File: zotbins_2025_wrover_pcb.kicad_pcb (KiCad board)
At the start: 2 copper layers, 107 x 98 mm, 26 parts

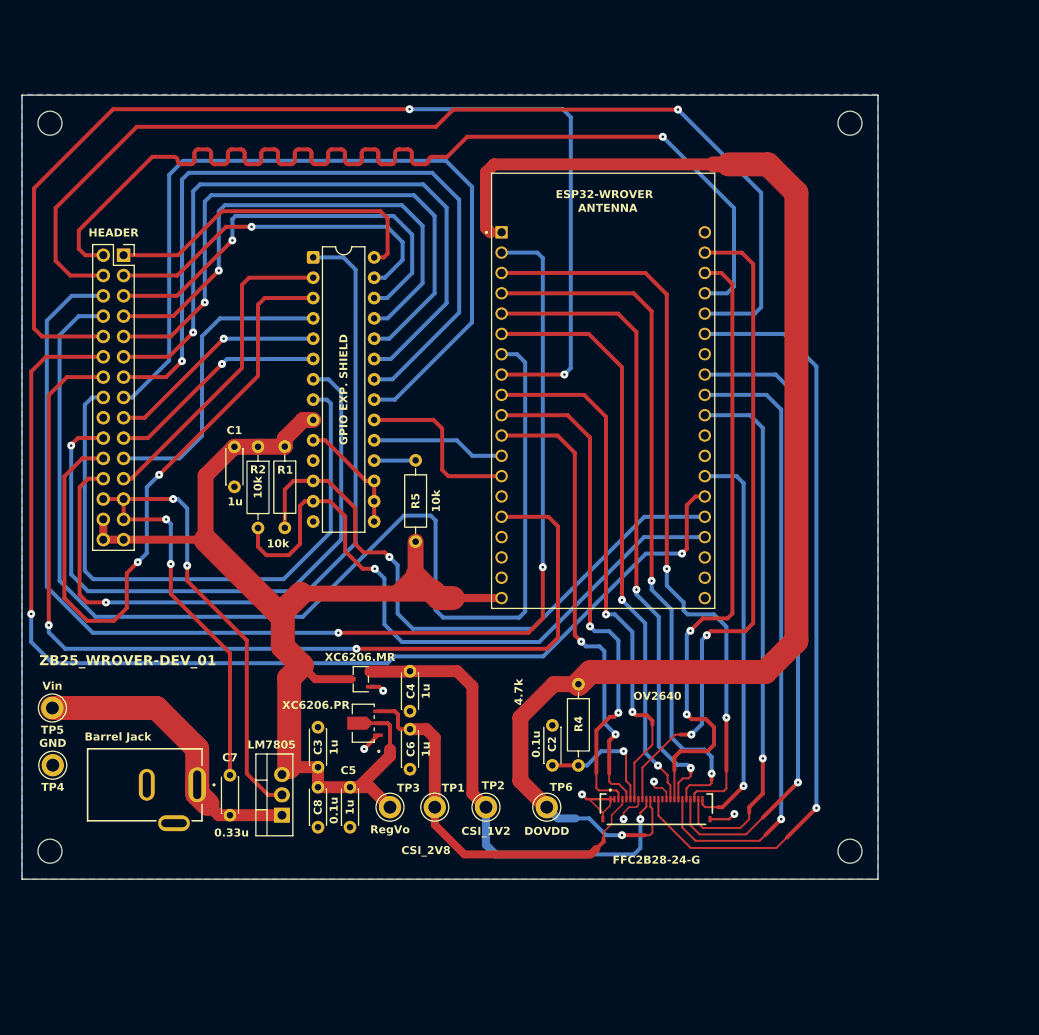
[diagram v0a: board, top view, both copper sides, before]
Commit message: basically the final version; just final adjustments with labeling and silkscreen needed. Traces, all components are all set.
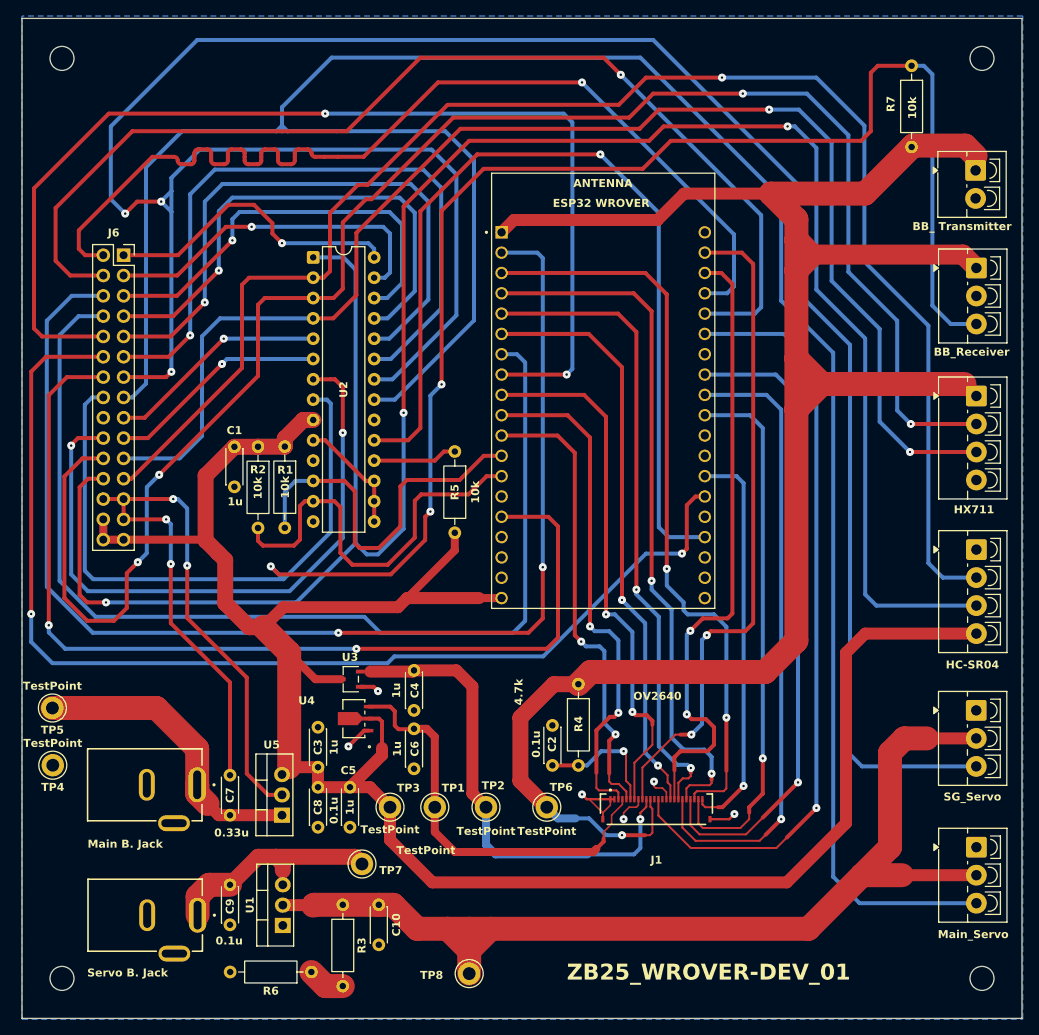
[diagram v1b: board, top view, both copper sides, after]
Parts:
- added BB_ Transmitter: BB_Transmitter_Screw_Terminal_01x02, TerminalBlock_4Ucon:TerminalBlock_4Ucon_1x02_P3.50mm_Vertical, F.Cu at (212.2, 56.4)
- added BB_Receiver: BB_Receiver_Screw_Terminal_01x03, TerminalBlock_4Ucon:TerminalBlock_4Ucon_1x03_P3.50mm_Vertical, F.Cu at (212.3, 68.6)
- added C10: 1u, Capacitor_THT:C_Disc_D4.3mm_W1.9mm_P5.00mm, F.Cu at (137.6, 148.2)
- added C9: 0.1u, Capacitor_THT:C_Disc_D4.3mm_W1.9mm_P5.00mm, F.Cu at (119.0, 145.7)
- added HC-SR04: HC-SR04_Screw_Terminal_01x04, TerminalBlock_4Ucon:TerminalBlock_4Ucon_1x04_P3.50mm_Vertical, F.Cu at (212.3, 103.8)
- added HX711: HX711_Screw_Terminal_01x04, TerminalBlock_4Ucon:TerminalBlock_4Ucon_1x04_P3.50mm_Vertical, F.Cu at (212.3, 84.6)
- added Main_Servo: Main_Servo_Screw_Terminal_01x03, TerminalBlock_4Ucon:TerminalBlock_4Ucon_1x03_P3.50mm_Vertical, F.Cu at (212.3, 141.0)
- added R3: 240, Resistor_THT:R_Axial_DIN0207_L6.3mm_D2.5mm_P10.16mm_Horizontal, F.Cu at (133.1, 148.2)
- added R6: 800, Resistor_THT:R_Axial_DIN0207_L6.3mm_D2.5mm_P10.16mm_Horizontal, F.Cu at (129.2, 156.6)
- added R7: 10k, Resistor_THT:R_Axial_DIN0207_L6.3mm_D2.5mm_P10.16mm_Horizontal, F.Cu at (204.2, 43.3)
- added SG_Servo: SG_Servo_Screw_Terminal_01x03, TerminalBlock_4Ucon:TerminalBlock_4Ucon_1x03_P3.50mm_Vertical, F.Cu at (212.3, 123.9)
- added Servo B. Jack: DCJ200-10-A-XX-K_REVA, Library:GCT_DCJ200-10-A-XX-K_REVA, F.Cu at (108.4, 149.5)
- added TP7: TestPoint, TestPoint:TestPoint_Keystone_5005-5009_Compact, F.Cu at (135.5, 143.1)
- added TP8: TestPoint, TestPoint:TestPoint_Keystone_5005-5009_Compact, F.Cu at (148.9, 156.8)
- added U1: LM350_TO220, Package_TO_SOT_THT:TO-220-3_Vertical, F.Cu at (125.6, 150.8)
- ESP32 WROVER: renamed from ESP32-WROVER
- Main B. Jack: renamed from Barrel Jack; value J2 -> DCJ200-10-A-XX-K_REVA
- TP1: value CSI_2V8 -> TestPoint
- TP2: value CSI_1V2 -> TestPoint
- TP3: value RegVo -> TestPoint
- TP4: value GND -> TestPoint
- TP5: value Vin -> TestPoint
- TP6: value DOVDD -> TestPoint
- U2: renamed from GPIO EXP. SHIELD
- moved R5 5.02 mm to (147.1, 91.5)
- moved U4 1.31 mm to (134.5, 124.9)
- moved U3 1.25 mm to (134.1, 120.0)
- moved C4 0.51 mm to (142.0, 118.9)
- moved C6 0.50 mm to (142.0, 126.2)
- renumbered FFC2B28-24-G to J1, HEADER to J6, XC6206.MR to U3, XC6206.PR to U4, LM7805 to U5
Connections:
- net /GPA0 renamed /MAIN_SERVO_PWM
- net /GPA1 renamed /SG_SERVO_PWM
- ESP32 WROVER pad J2-12: /MCP_INTB -> /GPIO_SDA
- ESP32 WROVER pad J2-13: /MCP_INTA -> /GPIO_SCK
- ESP32 WROVER pad J3-15: /GPIO_SDA -> unconnected-(U6-IO2-PadJ3-15)
- ESP32 WROVER pad J3-16: /GPIO_SCK -> /MCP_INTB
- U2 pad 20: /MCP_INTA -> unconnected-(U2-INTA-Pad20)
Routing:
- net /SG_SERVO_PWM: track 95.3 -> 308.6 mm, vias 1 -> 3
- net /MAIN_SERVO_PWM: track 103.9 -> 295.5 mm
- net /TRIG: track 95.0 -> 272.9 mm, vias 1 -> 3
- net /IR: track 75.5 -> 250.2 mm, vias 0 -> 3
- net /ECHO: track 40.2 -> 191.0 mm, vias 0 -> 1
- net /DT: track 38.2 -> 171.2 mm, vias 0 -> 2
- net +5V5: track 0.00 -> 132.2 mm
- net /SCK: track 82.6 -> 214.6 mm, vias 2 -> 4
- net +5V: track 151.3 -> 260.2 mm
- net /MCP_INTB: track 16.7 -> 114.8 mm, vias 0 -> 1
- net +3V3: track 176.0 -> 249.1 mm
- net /GPIO_SCK: track 82.8 -> 51.0 mm, vias 1 -> 0
- net /GPIO_SDA: track 77.6 -> 47.4 mm, vias 1 -> 0
- net Net-(U1-VI): track 0.00 -> 29.2 mm
- net /MCP_INTA: track 21.9 -> 0.00 mm
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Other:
- board size 107 x 98 mm -> 125 x 125 mm
